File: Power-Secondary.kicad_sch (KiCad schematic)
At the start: 0 parts

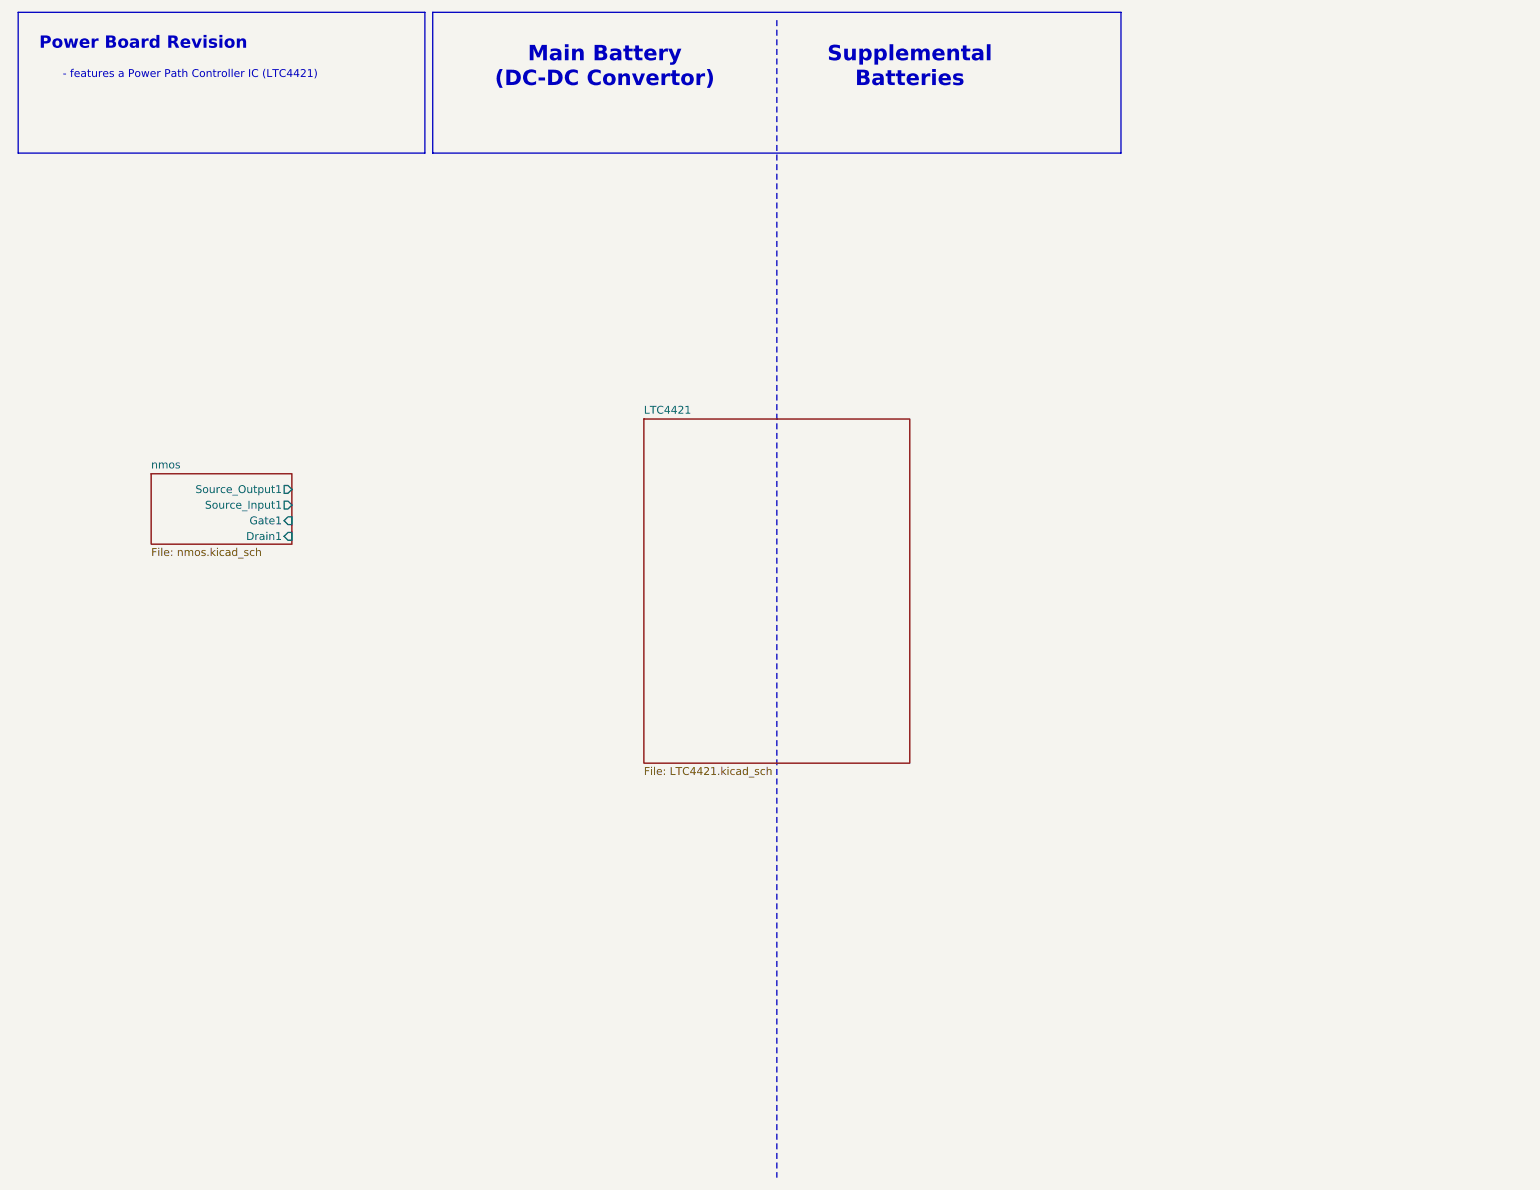
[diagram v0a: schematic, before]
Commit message: Finished sch
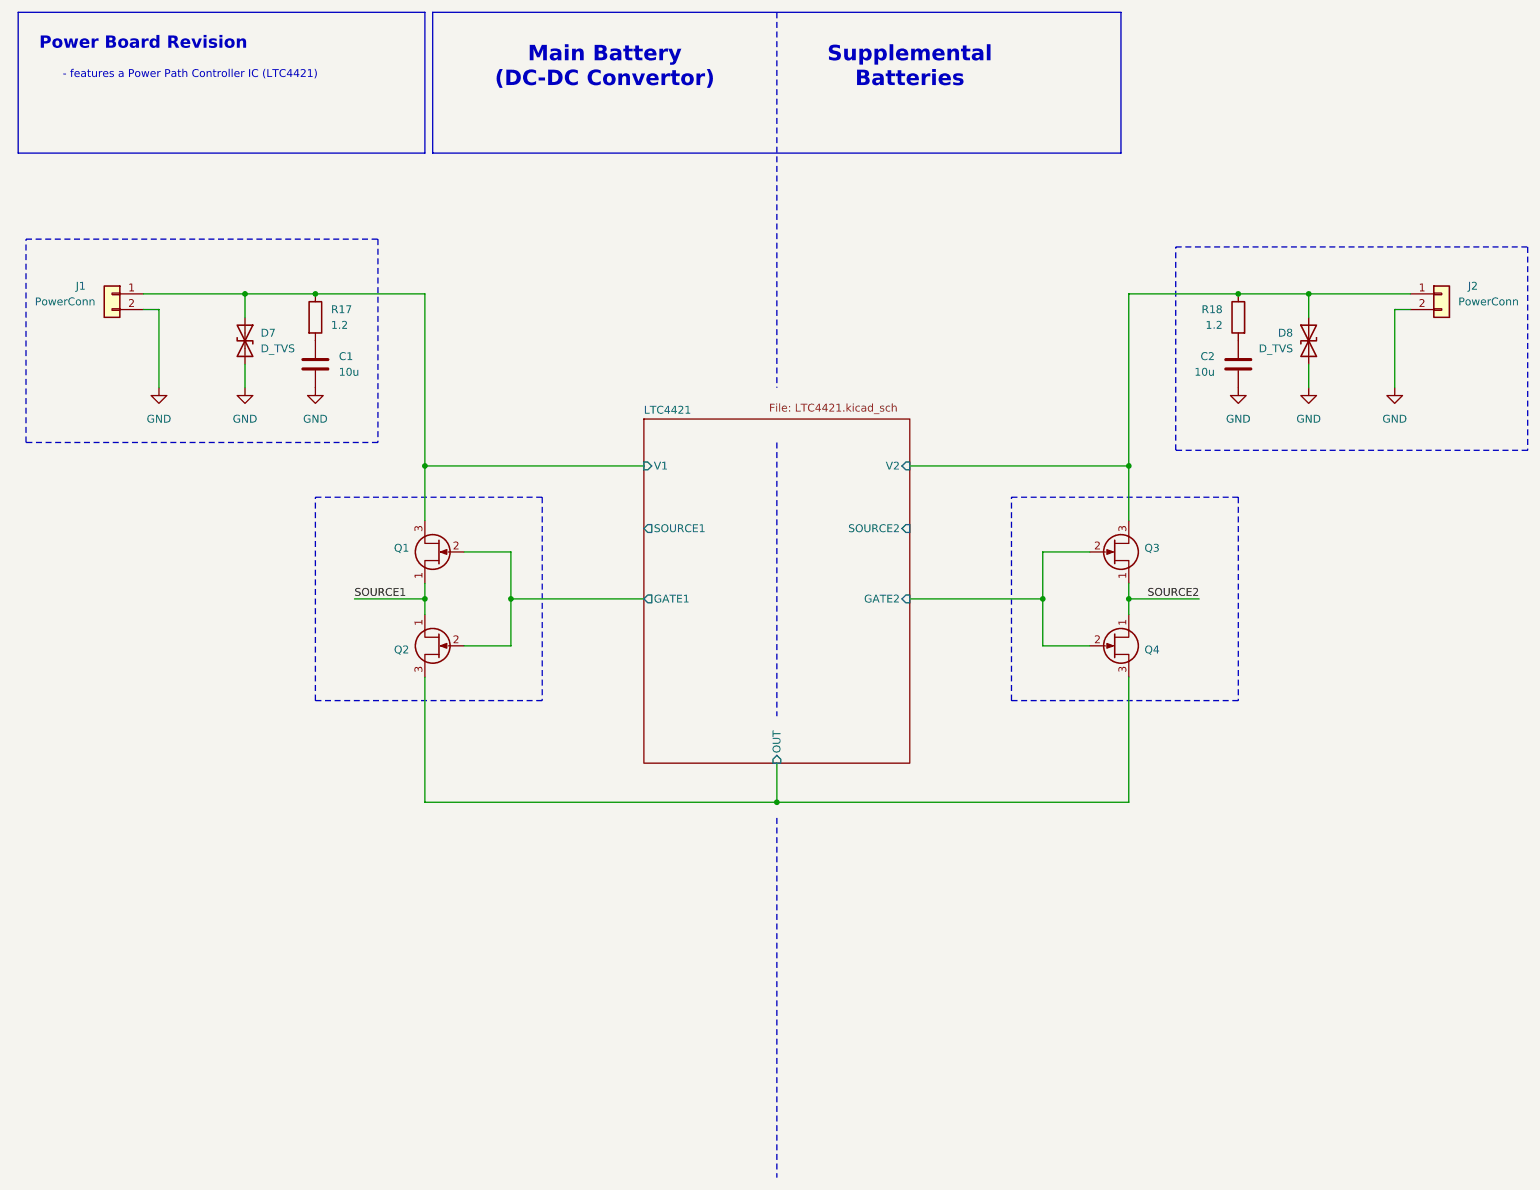
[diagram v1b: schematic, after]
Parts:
- added C1, C2: 10u, ECE319K:C_Axial_200mil, symbol ECE319K:C
- added D7, D8: D_TVS, symbol Device:D_TVS
- added J1, J2: PowerConn, UTSVT_Connectors:Molex_MicroFit3.0_1x2xP3.00mm_PolarizingPeg_Vertical, symbol Connector_Generic:Conn_01x02
- added Q1, Q2, Q3, Q4: ~, symbol Power-Board:SQJQ142E-T1_GE3
- added R17, R18: 1.2, symbol Device:R
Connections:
- new net: C1.1, R17.2
- new net: C2.1, R18.2
- new net GND: C1.2, C2.2, D7.2 (A2), D8.2 (A2), J1.2 (Pin_2), J2.2 (Pin_2)
- new net LTC4421/GATE1: Q1.2 (Gate), Q2.2 (Gate)
- new net LTC4421/GATE2: Q3.2 (Gate), Q4.2 (Gate)
- new net LTC4421/OUT: Q2.3 (Source), Q4.3 (Source)
- new net LTC4421/V1: D7.1 (A1), J1.1 (Pin_1), Q1.3 (Source), R17.1
- new net LTC4421/V2: D8.1 (A1), J2.1 (Pin_1), Q3.3 (Source), R18.1
- new net SOURCE1: Q1.1 (Drain), Q2.1 (Drain)
- new net SOURCE2: Q3.1 (Drain), Q4.1 (Drain)
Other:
- removed sheet nmos
- sheet LTC4421 ports: added GATE1, GATE2, OUT, SOURCE1, SOURCE2, V1, V2; removed none
